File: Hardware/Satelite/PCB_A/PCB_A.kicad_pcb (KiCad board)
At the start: 2 copper layers, 47 x 47 mm, 40 parts, among them J1 Batería LiPo (Soldada), J2 CONUFL001-SMD, J3 Servo Globo, J4 Conector_PCB_A-B, J5 Servo Paracaídas, Q1 SSM3J338R,LF, SW1 JS102011SAQN, U1 A2235-H, U2 CC1101RGP, U3 0915BM15A0001E, Y1 26 MHz

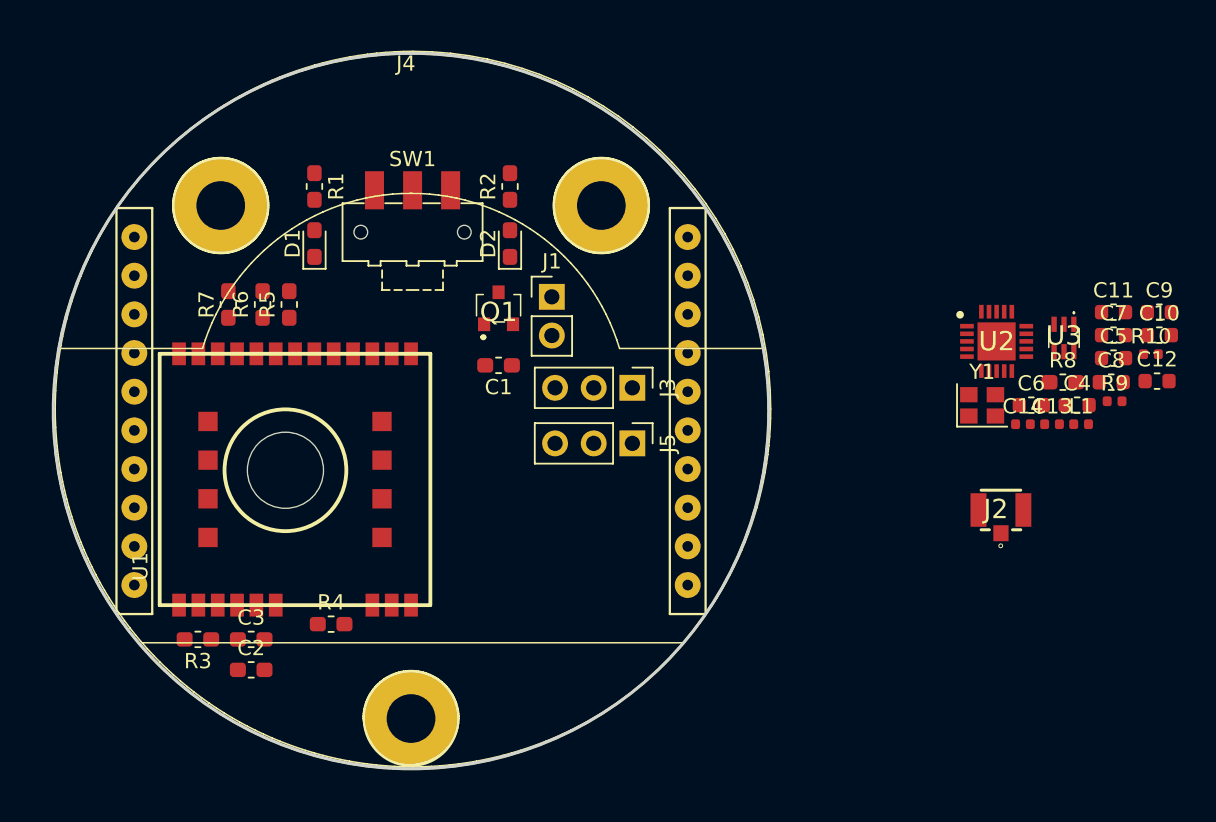
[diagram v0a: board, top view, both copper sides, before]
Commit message: PCB_A mas cambios
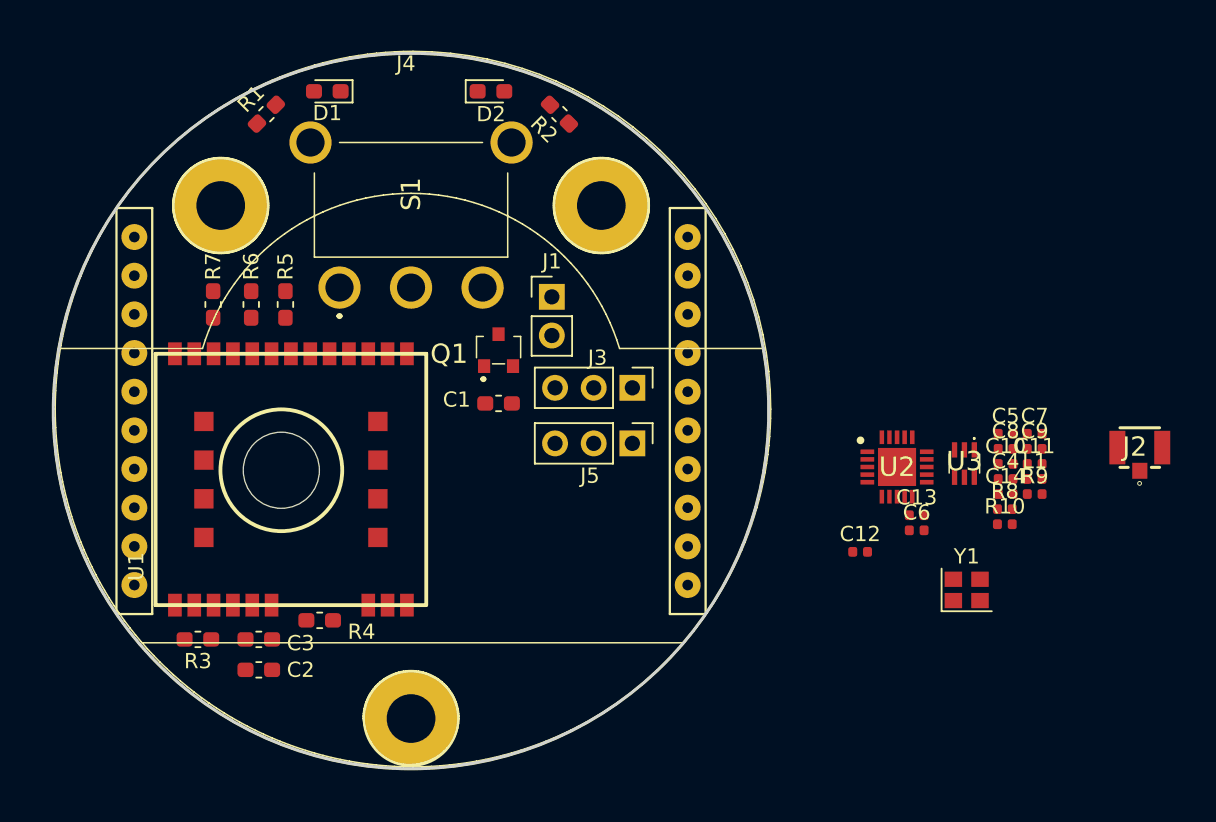
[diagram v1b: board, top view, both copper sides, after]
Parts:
- removed SW1: JS102011SAQN, Button_Switch_SMD:SW_SPDT_CK-JS102011SAQN
- added S1: 500SSP1S1M6QEA, SamacSys_Parts:500SSP1S1M6QEA, F.Cu at (0.00, -14.2)
- C10, C11, C12, C4, C5, C6, C7, C8, C9: footprint Capacitor_SMD:C_0603_1608Metric -> Capacitor_SMD:C_0402_1005Metric
- R8: footprint Resistor_SMD:R_0603_1608Metric_Pad1.05x0.95mm_HandSolder -> Resistor_SMD:R_0402_1005Metric
- moved C12 22.5 mm to (29.5, 9.25)
- moved R10 14.7 mm to (39.0, 7.44)
- moved C10 13.2 mm to (39.1, 3.48)
- moved Y1 12.2 mm to (36.5, 11.8)
- moved C9 12.2 mm to (41.0, 2.49)
- moved C11 11.2 mm to (41.0, 3.48)
- moved C6 11.1 mm to (33.2, 7.84)
- moved C13 10.7 mm to (33.2, 6.85)
- moved U2 10.5 mm to (31.9, 3.68)
- moved U3 10.5 mm to (36.4, 3.45)
- moved D2 10.1 mm to (5.25, -21.0), turned to 0 degrees
- moved D1 10.0 mm to (-5.50, -21.0), turned to 180 degrees
- moved J2 10.00 mm to (47.9, 2.40)
- moved R8 9.17 mm to (39.0, 6.45)
- moved C5 8.66 mm to (39.1, 1.50)
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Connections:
- U2 pad 2: /CC1101/SO -> /SDO
- U2 pad 20: /CC1101/SI -> /SDI
- U2 pad 7: GND -> /CS

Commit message: PCB_A terminado
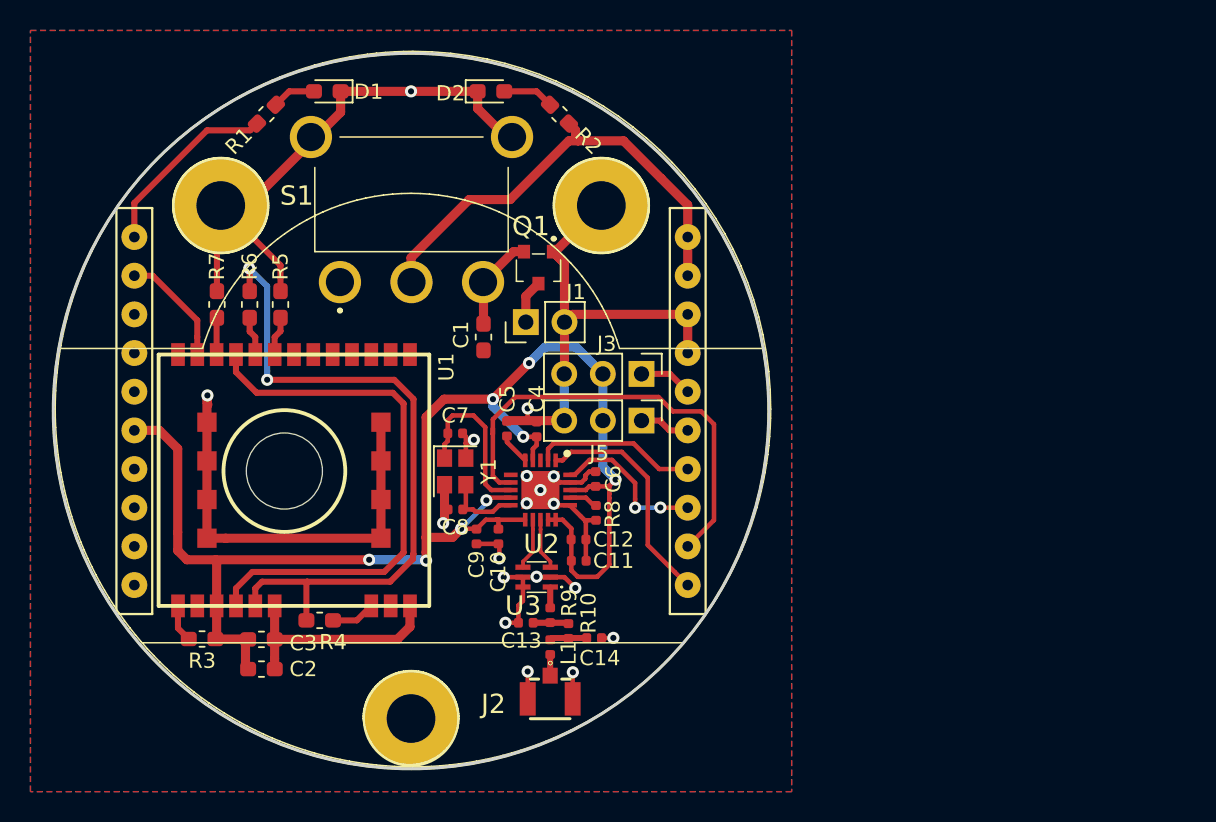
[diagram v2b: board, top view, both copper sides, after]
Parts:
- moved J2 42.1 mm to (9.14, 18.9), turned to 180 degrees
- moved C7 38.1 mm to (2.90, 1.47)
- moved C9 37.1 mm to (4.30, 8.24), turned to 270 degrees
- moved C8 36.4 mm to (2.92, 6.46), turned to 180 degrees
- moved Y1 34.5 mm to (2.90, 3.96), turned to 270 degrees
- moved L1 33.7 mm to (9.14, 15.5), turned to 270 degrees
- moved C10 33.7 mm to (5.74, 8.24), turned to 270 degrees
- moved R9 32.8 mm to (9.14, 13.4), turned to 270 degrees
- moved C5 32.8 mm to (6.30, 1.16), turned to 90 degrees
- moved C4 31.0 mm to (8.25, 1.21), turned to 90 degrees
- moved C11 30.6 mm to (11.0, 9.84)
- moved R10 29.5 mm to (10.3, 14.4), turned to 270 degrees
- moved U3 29.1 mm to (8.25, 10.9), turned to 270 degrees
- moved C14 28.6 mm to (12.0, 14.9)
- moved R8 26.9 mm to (12.2, 6.69), turned to 90 degrees
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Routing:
- net GND: track 0.00 -> 145.3 mm, vias 0 -> 18
- net +3V3_Internal: track 0.00 -> 100.7 mm, vias 0 -> 8
- net /GPS/GPS_1V8: track 0.00 -> 45.0 mm, vias 0 -> 2
- net Net-(U1-Pad19): track 0.00 -> 35.9 mm
- net Net-(J4-Pad1): track 0.00 -> 31.1 mm
- net /CS: track 0.00 -> 30.4 mm
- net /SCLK: track 0.00 -> 15.1 mm
- net /P1: track 0.00 -> 12.5 mm
- net Net-(C7-Pad1): track 0.00 -> 11.1 mm
- net /SDO: track 0.00 -> 10.8 mm
- net /SDI: track 0.00 -> 10.4 mm, vias 0 -> 2
- net /GPS_TX: track 0.00 -> 7.60 mm
- net +BATT: track 0.00 -> 6.85 mm
- net Net-(C8-Pad1): track 0.00 -> 5.10 mm
- net /S_GLOBO: track 0.00 -> 3.52 mm
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- added copper zone on B.Cu, net GND
- added copper zone on F.Cu, net GND
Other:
- net class ANT added: clearance 0.2, trace_width 0.4, via_dia 0.8, via_drill 0.4
- net class Alimentacion added: clearance 0.2, trace_width 0.3, via_dia 0.8, via_drill 0.4
- net class Default: trace_width 0.25 -> 0.3
- net class RF_DIF added: clearance 0.2, trace_width 0.25, via_dia 0.8, via_drill 0.4
